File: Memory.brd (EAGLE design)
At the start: 106.7 x 37.8 mm, 8 parts, among them IC1 AT28C256ZIF, IC2 HM62256DIP

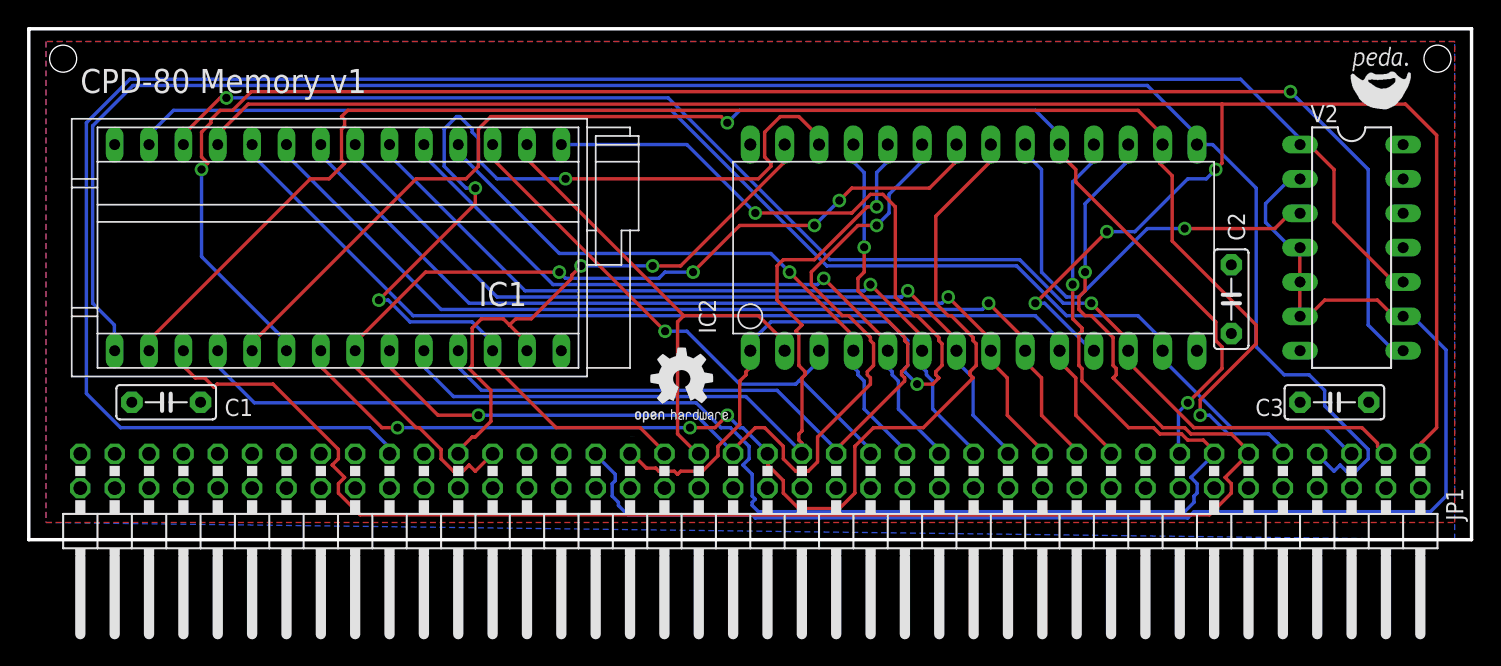
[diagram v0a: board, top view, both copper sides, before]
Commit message: Fix memory mapping issues
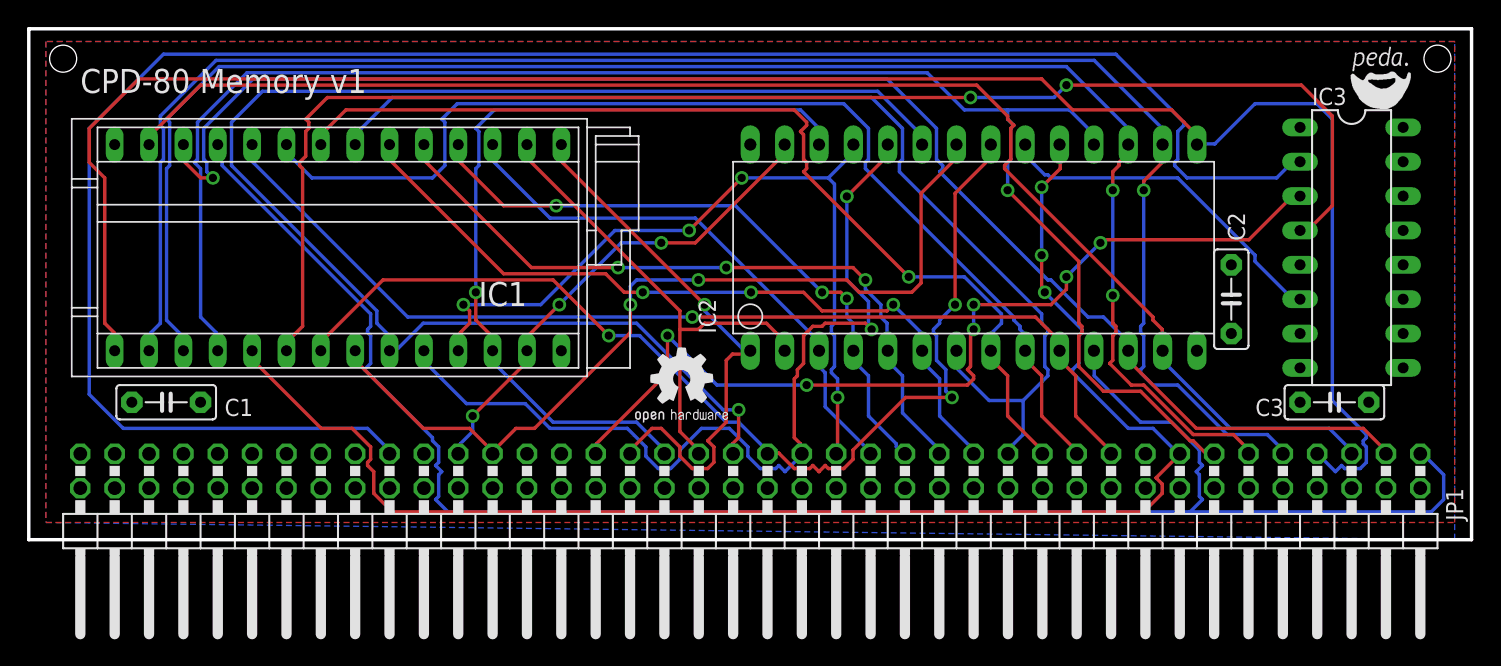
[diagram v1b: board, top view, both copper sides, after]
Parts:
- removed V2: 74HC00N, 74ttl-din:DIL14
- added IC3: 74LS139N, 74xx-eu:DIL16
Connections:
- removed net N$9: IC2.20, V2.3
- new net N$1: IC2.20, IC3.6
- net !MREQ: now also IC3.2; no longer V2.1, V2.10
- net A15: now also IC3.3; no longer V2.2, V2.4, V2.5, V2.6, V2.9
- net GND: now also IC3.1, IC3.8; no longer V2.7
- net N$2: now also IC3.4; no longer V2.8
- net VCC: now also IC3.16; no longer V2.14
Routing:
- net A11: track 70.7 -> 108.5 mm, vias 2 -> 1
- net A14: track 77.7 -> 40.6 mm, vias 2 -> 1
- net A15: track 103.7 -> 69.1 mm, vias 0 -> 6
- net N$9: track 32.5 -> 0.00 mm, vias 1 -> 0
- net N$1: track 0.00 -> 25.8 mm
- net A3: track 61.4 -> 80.7 mm, vias 1 -> 0
- net A13: track 80.2 -> 61.4 mm, vias 3 -> 1
- net N$2: track 124.0 -> 105.7 mm
- net D0: track 145.1 -> 130.9 mm, vias 3 -> 0
- net !MREQ: track 152.0 -> 143.0 mm
- net A1: track 71.5 -> 80.4 mm, vias 1 -> 0
- net D4: track 119.2 -> 127.8 mm
- net D1: track 102.9 -> 111.1 mm, vias 2 -> 1
- net D7: track 100.3 -> 108.4 mm, vias 2 -> 3
- net D3: track 137.8 -> 146.0 mm
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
